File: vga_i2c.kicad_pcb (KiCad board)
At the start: 2 copper layers, 87.9 x 77.2 mm, 34 parts, among them J1 VGA DB15 Female, J3 Atari 2600 Joystick DB9, J4 Conn_01x06, J5 Jumpers, J6 Conn_01x13, J7 VGA DB15 Female, SW1 SW_Push, SW2 SW_Push, SW3 SW_Push, SW4 SW Up, SW5 SW Down, SW6 SW Left, SW7 SW Right, SW8 SW Trigger, U1 MCP23017_SP

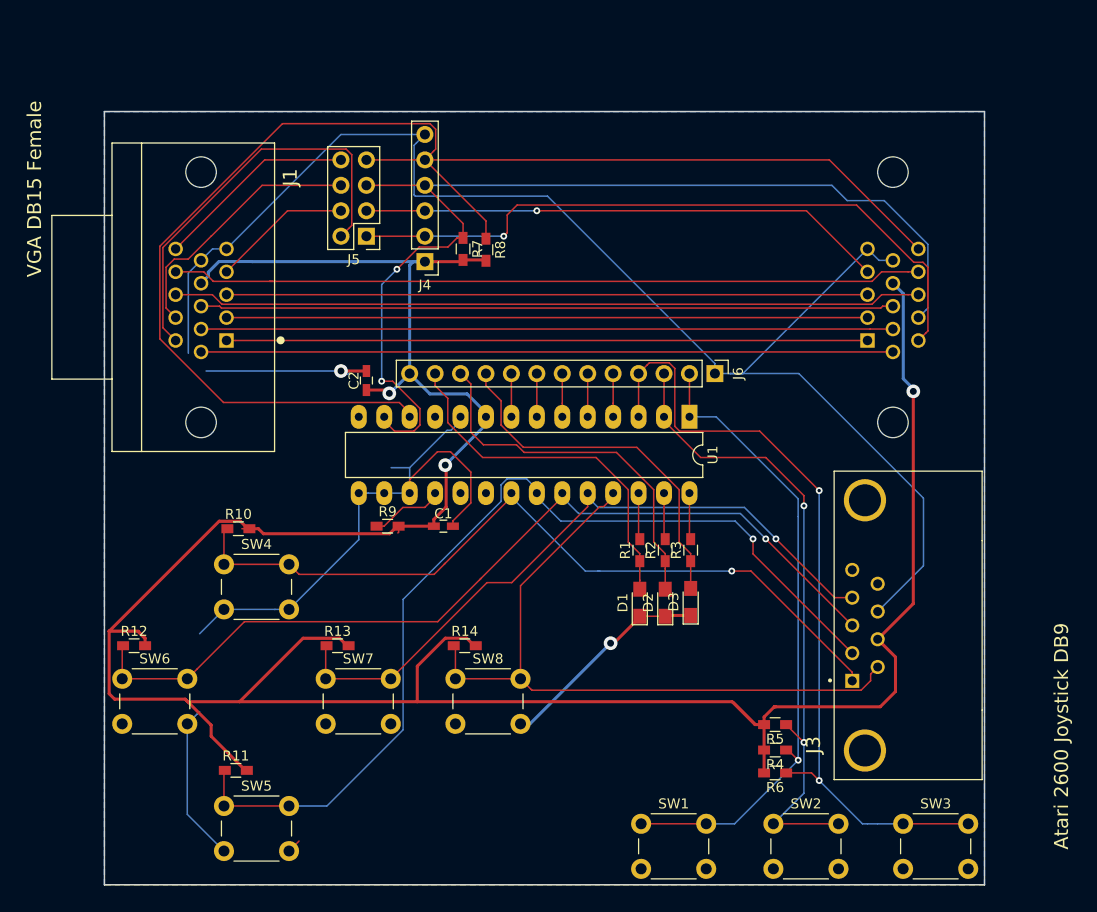
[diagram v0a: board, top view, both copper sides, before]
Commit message: !st production version.
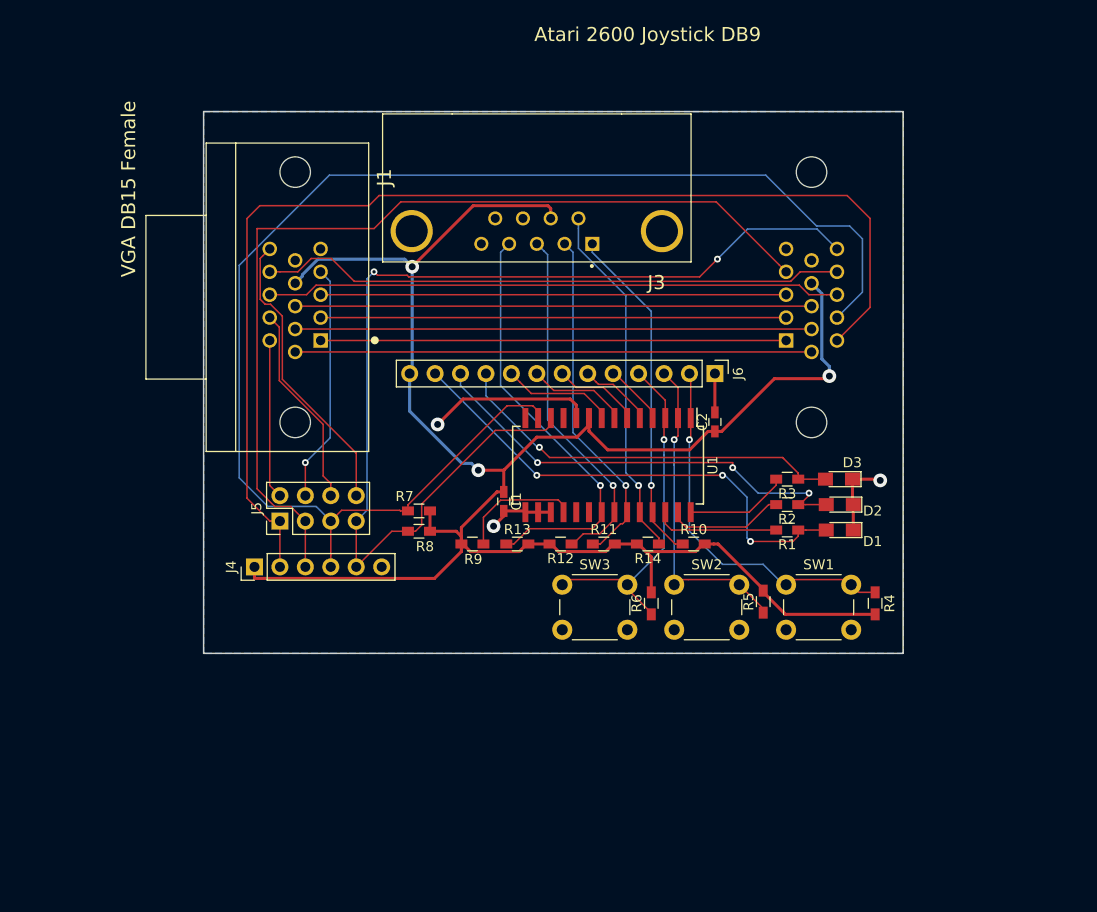
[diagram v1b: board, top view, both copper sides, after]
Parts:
- removed SW4: SW Up, Buttons_Switches_ThroughHole:SW_PUSH_6mm
- removed SW5: SW Down, Buttons_Switches_ThroughHole:SW_PUSH_6mm
- removed SW6: SW Left, Buttons_Switches_ThroughHole:SW_PUSH_6mm
- removed SW7: SW Right, Buttons_Switches_ThroughHole:SW_PUSH_6mm
- removed SW8: SW Trigger, Buttons_Switches_ThroughHole:SW_PUSH_6mm
- U1: value MCP23017_SP -> MCP23017_SO; footprint Housings_DIP:DIP-28_W7.62mm_LongPads -> Housings_SOIC:SOIC-28W_7.5x18.7mm_Pitch1.27mm
- moved J3 51.2 mm to (80.5, 65.8), turned to 180 degrees
- moved R10 45.5 mm to (96.2, 97.0)
- moved R12 43.8 mm to (82.9, 97.0), turned to 180 degrees
- moved R11 43.1 mm to (87.2, 97.0)
- moved SW3 41.6 mm to (83.1, 101.1)
- moved C2 35.0 mm to (98.3, 84.8)
- moved J4 34.9 mm to (52.3, 99.3), turned to 90 degrees
- moved J5 29.7 mm to (54.9, 94.7), turned to 90 degrees
- moved R8 28.9 mm to (68.8, 95.8), turned to 0 degrees
- moved SW1 27.9 mm to (105.4, 101.1)
- moved R7 26.5 mm to (68.8, 93.7), turned to 0 degrees
- moved SW2 25.8 mm to (94.2, 101.1)
- moved D1 21.2 mm to (110.8, 95.6), turned to 180 degrees
- moved R6 21.0 mm to (91.9, 103.0), turned to 90 degrees
- moved R14 20.9 mm to (91.6, 97.0), turned to 180 degrees
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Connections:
- net Net-(R9-Pad1) renamed /rstn
- U1 pad 21: /up -> /right
- U1 pad 22: /down -> /left
- U1 pad 23: /left -> /down
- U1 pad 24: /right -> /trigger
- U1 pad 25: /trigger -> /up
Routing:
- net GND: track 256.7 -> 35.0 mm, vias 2 -> 3
- net +5V: track 343.7 -> 197.7 mm
- net /down: track 97.0 -> 34.5 mm
- net /left: track 90.0 -> 36.0 mm
- net Net-(J6-Pad4): track 80.7 -> 34.2 mm, vias 2 -> 1
- net /rsvd0_m: track 68.7 -> 114.4 mm, vias 1 -> 0
- net /up: track 79.8 -> 34.2 mm
- net /rsvd2_m: track 52.6 -> 93.5 mm, vias 1 -> 0
- net /ddc_sda_m: track 104.0 -> 141.0 mm, vias 2 -> 0
- net /ddc_scl_m: track 143.2 -> 106.7 mm, vias 0 -> 2
- net /trigger: track 70.0 -> 35.8 mm, vias 0 -> 1
- net Net-(J6-Pad3): track 64.8 -> 32.4 mm, vias 2 -> 1
- net Net-(J6-Pad2): track 64.6 -> 36.7 mm
- net /right: track 69.3 -> 42.6 mm
- net /rsvd0_f: track 41.6 -> 15.9 mm
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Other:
- board size 87.9 x 77.2 mm -> 69.8 x 54.1 mm
